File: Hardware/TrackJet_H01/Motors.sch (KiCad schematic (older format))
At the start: 52 parts, among them J10 Conn_01x02, J11 Conn_01x02, J12 Conn_01x03_Male, J13 Conn_01x02, J14 Conn_01x02, J15 Conn_01x03_Male, J7 Conn_01x02, J8 Conn_01x03_Male, J9 Conn_01x02, Q6 AO3400A, Q7 AO3400A, Q8 AO3400A, Q9 AO3400A, U16 DRV8871DDA, U17 LM358, U18 DRV8871DDA, U19 LM358

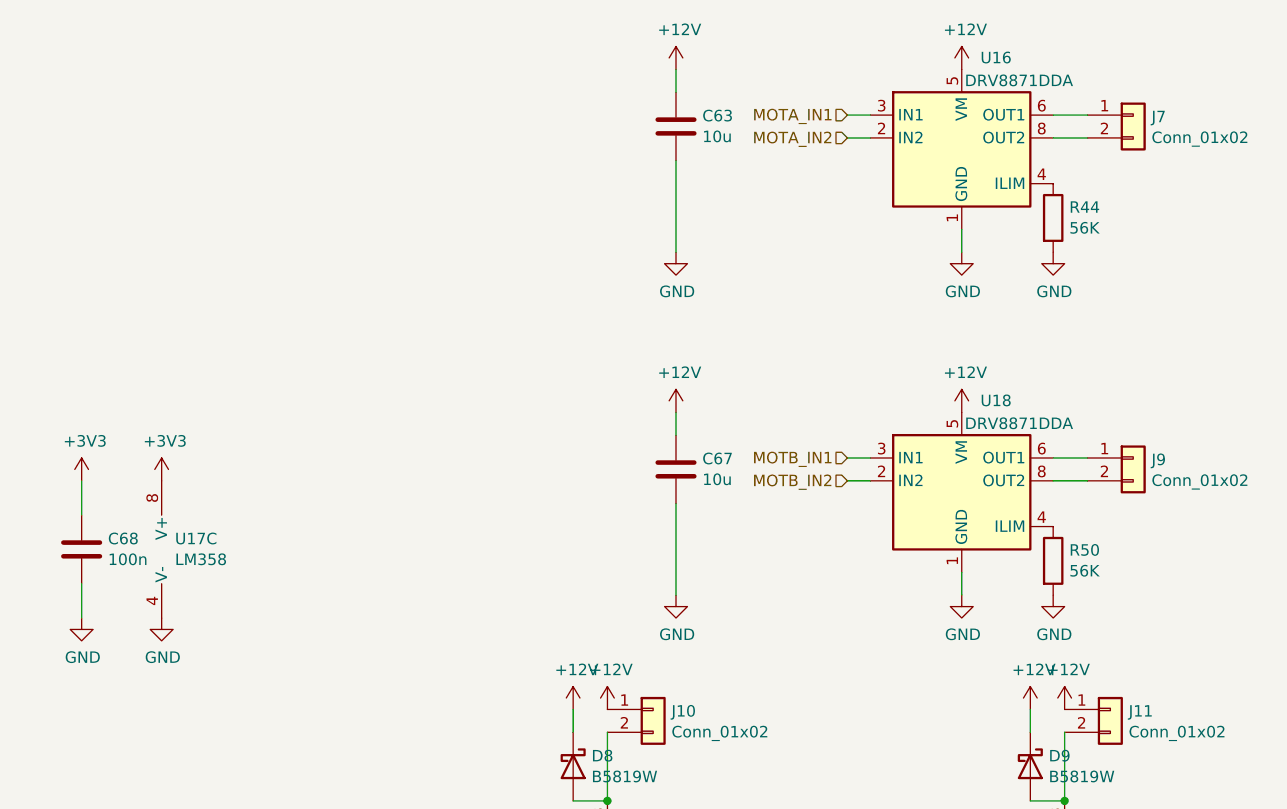
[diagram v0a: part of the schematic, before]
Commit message: H01 update
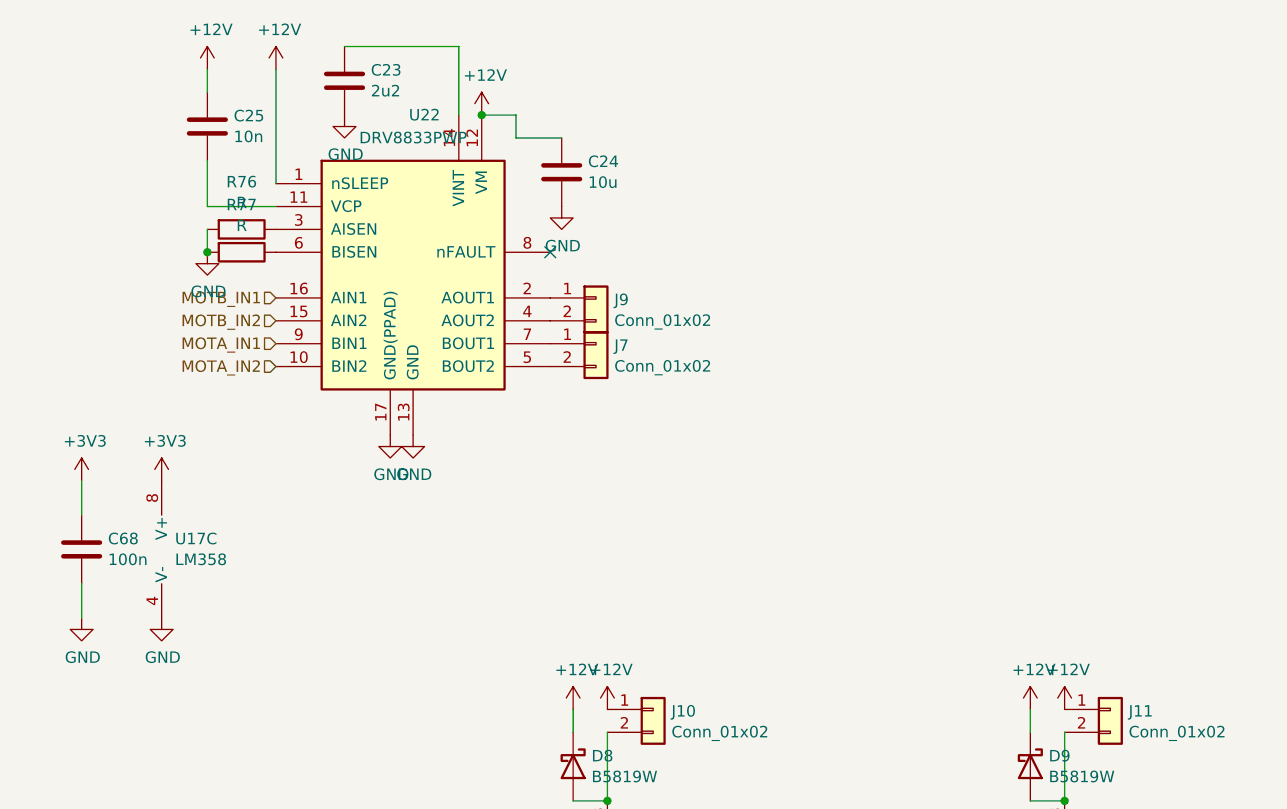
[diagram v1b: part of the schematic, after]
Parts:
- removed C63, C67: 10u, Capacitor_SMD:C_0805_2012Metric, symbol Device:C
- removed R44, R50: 56K, Resistor_SMD:R_0603_1608Metric, symbol Device:R
- removed U16, U18: DRV8871DDA, Package_SO:Texas_HTSOP-8-1EP_3.9x4.9mm_P1.27mm_EP2.95x4.9mm_Mask2.4x3.1mm_ThermalVias, symbol Driver_Motor:DRV8871DDA
- added C23: 2u2, Capacitor_SMD:C_0603_1608Metric, symbol Device:C
- added C24: 10u, Capacitor_SMD:C_0805_2012Metric, symbol Device:C
- added C25: 10n, Capacitor_SMD:C_0603_1608Metric, symbol Device:C
- added R76, R77: R, Resistor_SMD:R_1206_3216Metric_Pad1.30x1.75mm_HandSolder, symbol Device:R
- added U22: DRV8833PWP, Package_SO:HTSSOP-16-1EP_4.4x5mm_P0.65mm_EP3.4x5mm_Mask2.46x2.31mm_ThermalVias, symbol Driver_Motor:DRV8833PWP
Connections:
- net +12V: now also C24.1, C25.1, U22.1 (nSLEEP), U22.12 (VM)
- net GND: now also C23.2, C24.2, R76.2, R77.2, U22.13 (GND), U22.17 (GND(PPAD))
- net MOTA_IN1: now also U22.9 (BIN1)
- net MOTA_IN2: now also U22.10 (BIN2)
- net MOTB_IN1: now also U22.16 (AIN1)
- net MOTB_IN2: now also U22.15 (AIN2)
- net at J7.1 (Pin_1): now also U22.7 (BOUT1)
- net at J7.2 (Pin_2): now also U22.5 (BOUT2)
- net at J9.1 (Pin_1): now also U22.2 (AOUT1)
- net at J9.2 (Pin_2): now also U22.4 (AOUT2)
- new net: C25.2, U22.11 (VCP)
- new net: C23.1, U22.14 (VINT)
- new net: R76.1, U22.3 (AISEN)
- new net: R77.1, U22.6 (BISEN)
- no-connect marks 0 -> 1
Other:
- moved on the sheet: J7, J9
